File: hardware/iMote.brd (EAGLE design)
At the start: 43 x 50 mm, 55 parts, among them CN1 USB-MINIB-UX60SC-MB, CN2 ICSP, CN3 CC-HEADER, CN4 IRLED_Conn, CN5 PIN_Header, IC1 ATmega328P-AU, IC2 BLE112-A-VISUAL, IC3 FT232RLSSOP, Q1 16MHz, Q2 BSS138, T1 2SD1718

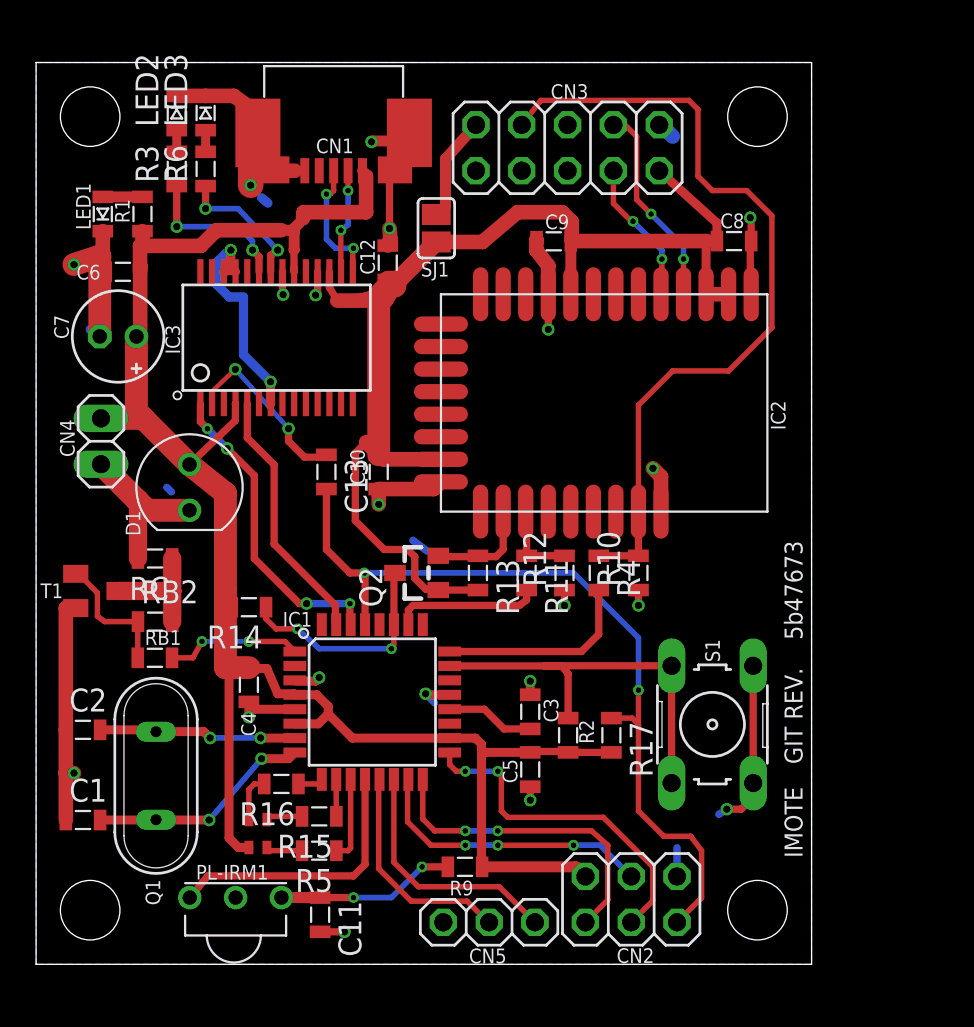
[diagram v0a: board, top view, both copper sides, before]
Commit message: 回路修正_暫定版です
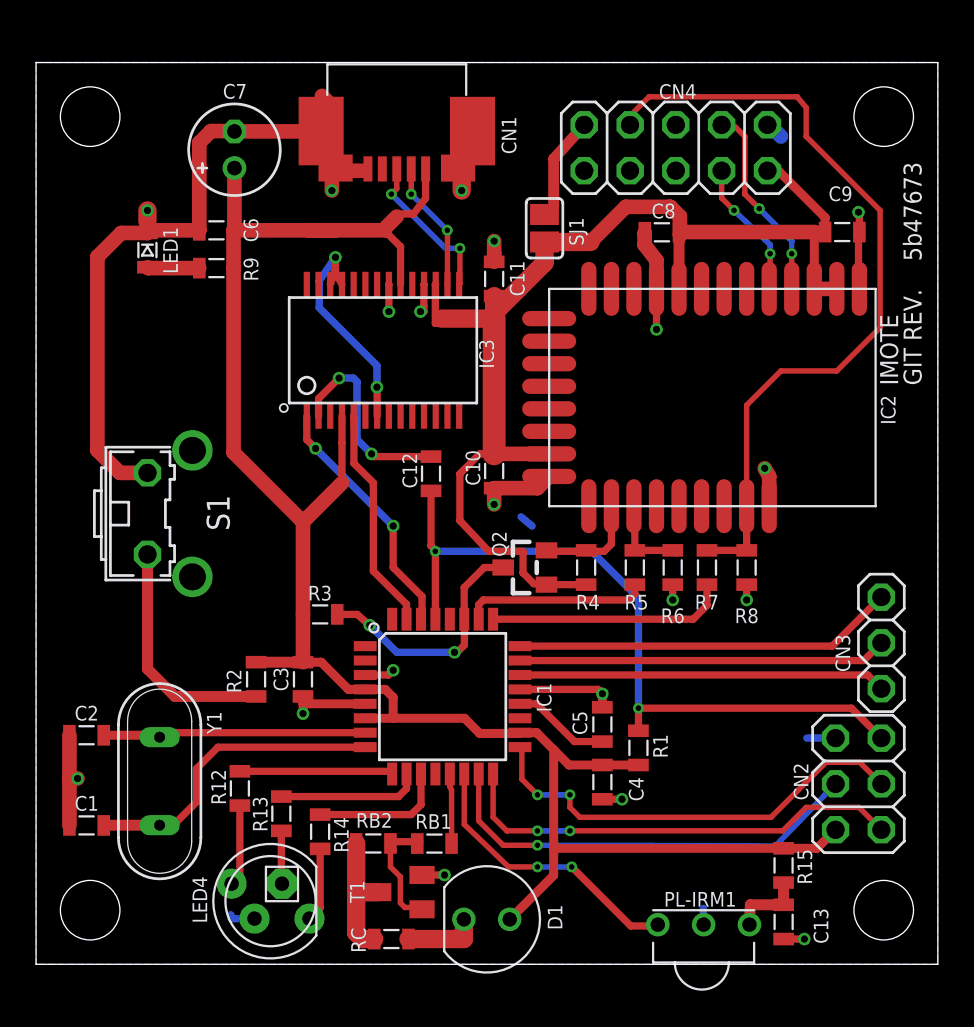
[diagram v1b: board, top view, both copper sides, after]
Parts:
- removed CN5: PIN_Header, my:PINHEAD-1X03
- removed LED2, LED3: 5V, my:LED-2012
- removed Q1: 16MHz, my:XTAL-HC-49/S
- removed R10: 3.3k, my:2012
- removed R11: 2.2k, my:2012
- removed R16: 750, my:2012
- removed R17: 1K, my:2012
- added R7: 2.2k, my:2012
- added R8: 3.3k, my:2012
- added Y1: 16MHz, my:XTAL-HC-49/S
- C11: value 4.7uF -> 0.1uF
- C13: value 0.1uF -> 4.7uF
- CN3: value CC-HEADER -> PIN_Header; device pinhead:2X05 -> my:PINHEAD-1X03
- CN4: value IRLED_Conn -> CC-HEADER; device pinhead:1X02 -> pinhead:2X05
- LED4: value OSTB0603C1C-A -> 5MMRGBLED; device FullColorLED:OSTB0603C1C -> adafruit:LED5MMRGB
- R1: value 330 -> 10K
- R12: value 3.3k -> 1.2K
- R13: value 4.7k -> 2.4k
- R14: value 10k -> 1k
- R15: value 820 -> 200
- R3: value 330 -> 10k
- R4: value 2.2k -> 4.7k
- R5: value 1K -> 2.2k
- R6: value 330 -> 3.3k
- R9: value 200 -> 220
- S1: value B3F-1000 -> S1; device switch-omron:B3F-10XX -> switch-omron:B3F-31XX
- moved R1 40.4 mm to (33.4, 12.0), turned to 270 degrees
- moved C11 36.5 mm to (25.4, 38.0), turned to 90 degrees
- moved R9 35.9 mm to (10.0, 38.6), turned to 180 degrees
- moved CN4 35.8 mm to (35.5, 45.3), turned to 180 degrees
- moved C13 35.6 mm to (41.5, 2.35)
- moved R6 34.0 mm to (35.3, 22.0)
- moved CN3 32.5 mm to (46.9, 17.8), turned to 90 degrees
- moved S1 32.3 mm to (7.42, 25.0), turned to 270 degrees
- moved D1 29.1 mm to (25.0, 2.49), turned to 180 degrees
- moved PL-IRM1 26.0 mm to (37.0, 2.20)
- moved R3 25.9 mm to (15.8, 19.4), turned to 180 degrees
- moved R15 25.9 mm to (41.4, 5.48), turned to 90 degrees
- moved RC 24.8 mm to (19.7, 1.40), turned to 0 degrees
- moved T1 23.7 mm to (20.2, 4.00), turned to 90 degrees
- moved R5 23.5 mm to (33.2, 22.0), turned to 270 degrees
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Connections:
- removed net A0/BTN: IC1.23, R2.1, S1.1, S1.2
- removed net A1/RST_HV: IC1.24, R4.2
- removed net D10: CN5.3, IC1.14
- removed net D5/LED_B: IC1.9, R16.1
- removed net D7/LED_R: IC1.11, R5.1
- removed net D9: CN5.2, IC1.13
- removed net N$4: LED2.A, R3.2
- removed net N$6: LED3.A, R6.2
- removed net USB/RXLED: IC3.22, R6.1
- removed net USB/TXLED: IC3.23, R3.1
- new net A0: CN3.2, IC1.23
- new net A1: CN3.3, IC1.24
- new net A2/BTN: R2.1, S1.2
- new net A2/RST_HV: IC1.25, R7.2
- new net A7: CN3.1, IC1.22
- new net D10/IRIN: IC1.14, PL-IRM1.1
- new net D2_BTN: IC1.32
- new net D5/LED_R: IC1.9, R12.1
- new net D7/LED_B: IC1.11, R14.1
- new net D9/IROUT: IC1.13, RB1.2
- net !BLE/RST: now also CN4.7, R7.1, R8.2; no longer CN3.7, R10.2, R4.1
- net !RESET: now also C12.2, R1.1; no longer C13.2, R17.1
- net +3V3: now also C11.1, CN4.2, R4.2; no longer C12.1, CN3.2, R13.2
- net +5V: now also C3.2, R1.2, R15.2, R3.2, R9.1; no longer C5.2, CN4.1, LED4.ANODE, R1.1, R14.2, R17.2, R9.2
- net A3/TX_HV: now also R5.2; no longer R11.2
- net A4/RX_HV: now also R3.1; no longer R14.1
- net AREF: now also C5.2; no longer C3.2
- net BLE/P2_1: now also CN4.4; no longer CN3.4
- net BLE/P2_2: now also CN4.3; no longer CN3.3
- net D3/IROUT: no longer RB1.2
- net D6/LED_G: now also R13.1; no longer R15.1
- net D8/IRIN: no longer PL-IRM1.1
- net GND: now also C13.2, CN4.1, LED4.3, R6.1, R8.1, S1.1; no longer C12.2, CN3.1, LED2.C, LED3.C, R10.1, R12.1, S1.3, S1.4
- net IRLED: no longer CN4.2
- net N$1: now also Y1.1; no longer Q1.1
- net N$15: now also LED4.2, R13.2; no longer LED4.GREEN, R15.2
- net N$16: now also C13.1, R15.1; no longer C11.1, R9.1
- net N$17: now also LED4.1, R14.2; no longer LED4.BLUE, R16.2
- net N$2: now also Y1.2; no longer Q1.2
- net N$3: now also R9.2; no longer R1.2
- net N$5: now also LED4.4, R12.2; no longer LED4.RED, R5.2
- net N$8: now also C12.1; no longer C13.1
- net PRG/VDD: now also CN4.9; no longer CN3.9
- net RX_LV/BLERX: now also R5.1, R6.2; no longer R11.1, R12.2
- net TX_LV/BLETX: now also R4.1; no longer R13.1
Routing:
- net A0/BTN: track 23.0 -> 0.00 mm
- net A1: track 0.00 -> 21.2 mm
- net A0: track 0.00 -> 20.4 mm
- net A7: track 0.00 -> 20.4 mm
- net D10/IRIN: track 0.00 -> 15.9 mm, vias 0 -> 2
- net D8/IRIN: track 15.3 -> 0.00 mm
- net D10: track 13.8 -> 0.00 mm
- net A2/RST_HV: track 0.00 -> 13.3 mm
- net A2/BTN: track 0.00 -> 13.0 mm
- net D9: track 12.3 -> 0.00 mm
- net A1/RST_HV: track 11.1 -> 0.00 mm
- net USB/TXLED: track 8.63 -> 0.00 mm, vias 2 -> 0
- net D5/LED_R: track 0.00 -> 8.50 mm
- net USB/RXLED: track 8.44 -> 0.00 mm, vias 2 -> 0
- net D11/MOSI: track 16.0 -> 24.4 mm, vias 3 -> 1
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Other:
- board size 43 x 50 mm -> 50 x 50 mm
